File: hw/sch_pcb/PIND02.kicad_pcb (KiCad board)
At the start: 2 copper layers, 40.1 x 40.1 mm, 56 parts, among them J1 Conn_Coaxial, J2 HEADER_2x05_PARALLEL, J3 HEADER_2x01, M1 HOLE M3, M2 HOLE M3, M3 HOLE, M4 HOLE, Q1 2SK2394-6, U1 OPA2314, U2 ISL21080DIH312Z-TK, U3 SHT31-DIS, U4 TPS613222ADBV

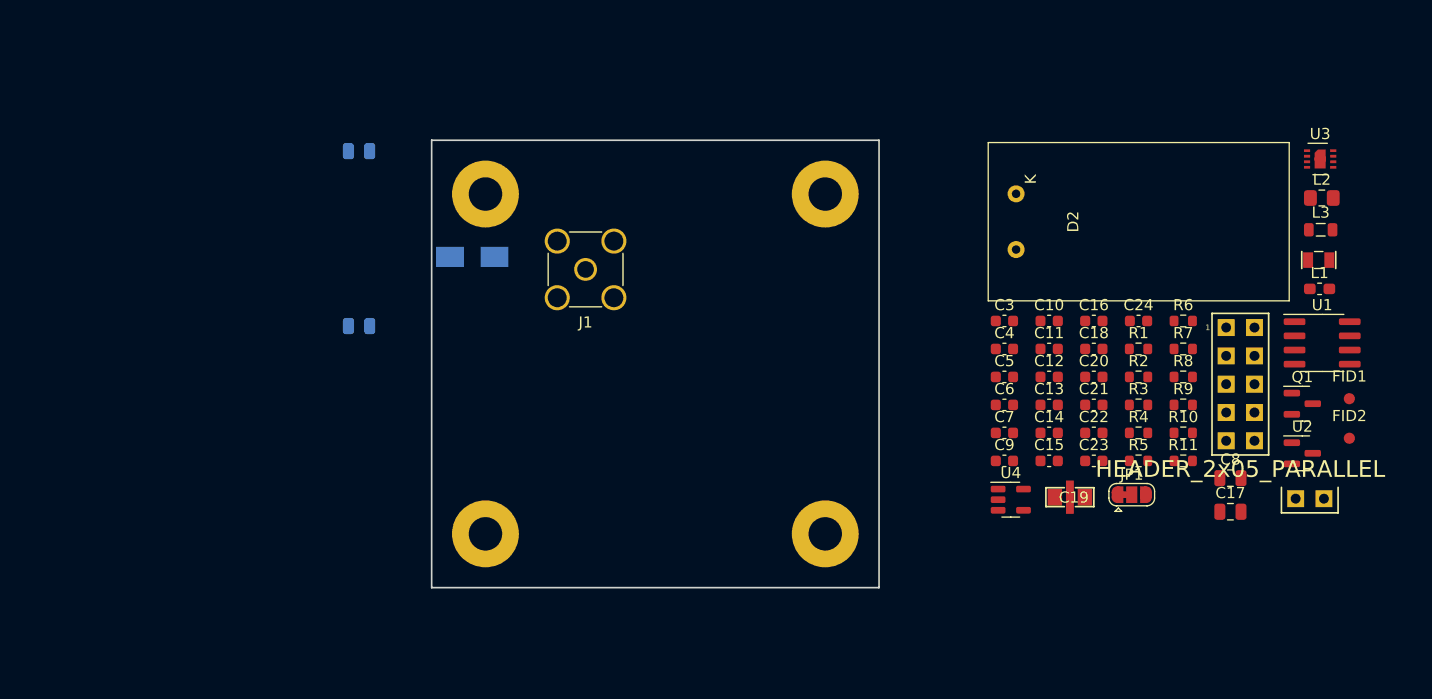
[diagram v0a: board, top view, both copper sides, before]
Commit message: PCB design WIP.
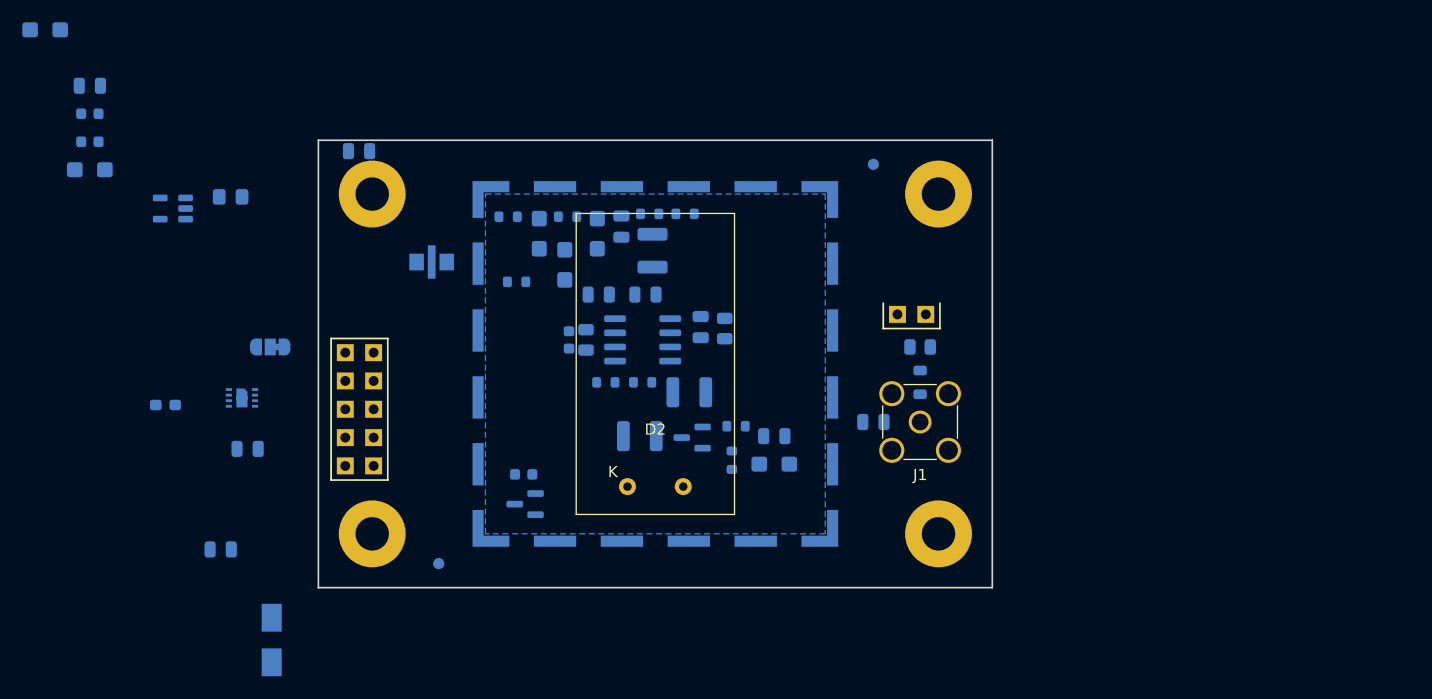
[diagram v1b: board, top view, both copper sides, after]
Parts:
- added M5: RFShield_TwoPieces, RF_Shielding:Laird_Technologies_BMI-S-204-F_32.00x32.00mm, B.Cu at (148.5, 105.0)
- C10, C23, C24, C4, C7, C9: footprint Capacitor_SMD:C_0603_1608Metric -> Capacitor_Tantalum_SMD:CP_EIA-3216-18_Kemet-A; moved to B.Cu
- C11, C13, C14, C20, C3, C6: footprint Capacitor_SMD:C_0603_1608Metric -> Capacitor_SMD:C_0805_2012Metric; moved to B.Cu
- C12, C15, C5: footprint Capacitor_SMD:C_0603_1608Metric -> Capacitor_SMD:C_1210_3225Metric; moved to B.Cu
- C16, C17, C18, C19, C21, C22, C8, FID1, FID2, JP1, L1, L2, L3, Q1, R1, R11, R2, R3, R5, R6, R7, R8, R9, U1, U2, U3, U4: moved to B.Cu
- J2: value HEADER_2x05_PARALLEL -> MLAB I2C interface
- R10, R4: footprint Resistor_SMD:R_0603_1608Metric -> Resistor_SMD:R_0805_2012Metric; moved to B.Cu
- R12: footprint Mlab_R:SMD-0805 -> Resistor_SMD:R_0805_2012Metric; moved to B.Cu
- moved L1 104.0 mm to (104.6, 108.7), turned to 180 degrees
- moved C24 101.5 mm to (93.8, 75.0), turned to 180 degrees
- moved U3 99.1 mm to (111.4, 108.0), turned to 180 degrees
- moved L2 97.9 mm to (110.4, 90.0), turned to 180 degrees
- moved C20 93.8 mm to (97.8, 80.0), turned to 180 degrees
- moved C21 93.8 mm to (97.8, 82.6), turned to 180 degrees
- moved C22 93.8 mm to (97.8, 85.1), turned to 180 degrees
- moved C23 93.8 mm to (97.8, 87.6), turned to 180 degrees
- moved C17 88.3 mm to (111.9, 112.6), turned to 180 degrees
- moved FID2 82.5 mm to (129.1, 122.9), turned to 180 degrees
- moved U4 79.6 mm to (105.2, 91.1), turned to 180 degrees
- moved J2 79.0 mm to (122.0, 109.1)
- moved JP1 78.4 mm to (114.0, 103.5), turned to 180 degrees
- moved U2 69.9 mm to (136.8, 117.6), turned to 180 degrees
- moved C19 61.0 mm to (128.4, 95.9), turned to 180 degrees
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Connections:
- C10 pad 2: GND -> GNDA
- C11 pad 2: GND -> GNDA
- C15 pad 2: GND -> GNDA
- C18 pad 2: GND -> GNDA
- C20 pad 2: GND -> GNDA
- C3 pad 2: GND -> GNDA
- C4 pad 2: GND -> GNDA
- C6 pad 2: GND -> GNDA
- C7 pad 2: GND -> GNDA
- C9 pad 2: GND -> GNDA
- R3 pad 2: GND -> GNDA
- U1 pad 4: GND -> GNDA
- U2 pad 3: GND -> GNDA
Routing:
- added copper zone on B.Cu, net GNDA
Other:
- board size 40.1 x 40.1 mm -> 60.5 x 40.1 mm
